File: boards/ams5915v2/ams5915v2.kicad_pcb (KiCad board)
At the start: 2 copper layers, 20 x 56.5 mm, 32 parts, among them J1 Conn_01x04, M3 MountingHole_3.2mm_M3, U1 TLV73333PDBVR, U2 MAX4995A, U3 AMS5915, U4 MAX4995A, U5 AMS5915

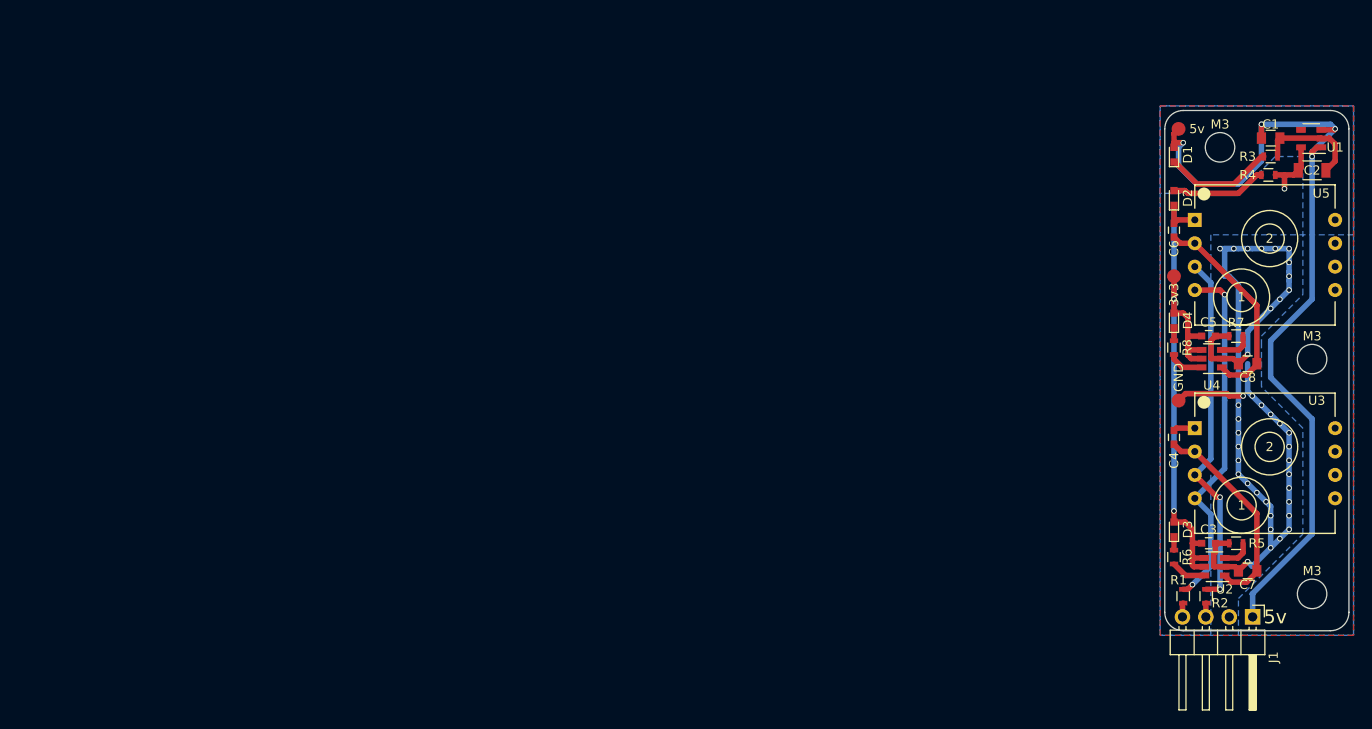
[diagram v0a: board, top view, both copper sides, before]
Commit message: [ams5915v2] new board design
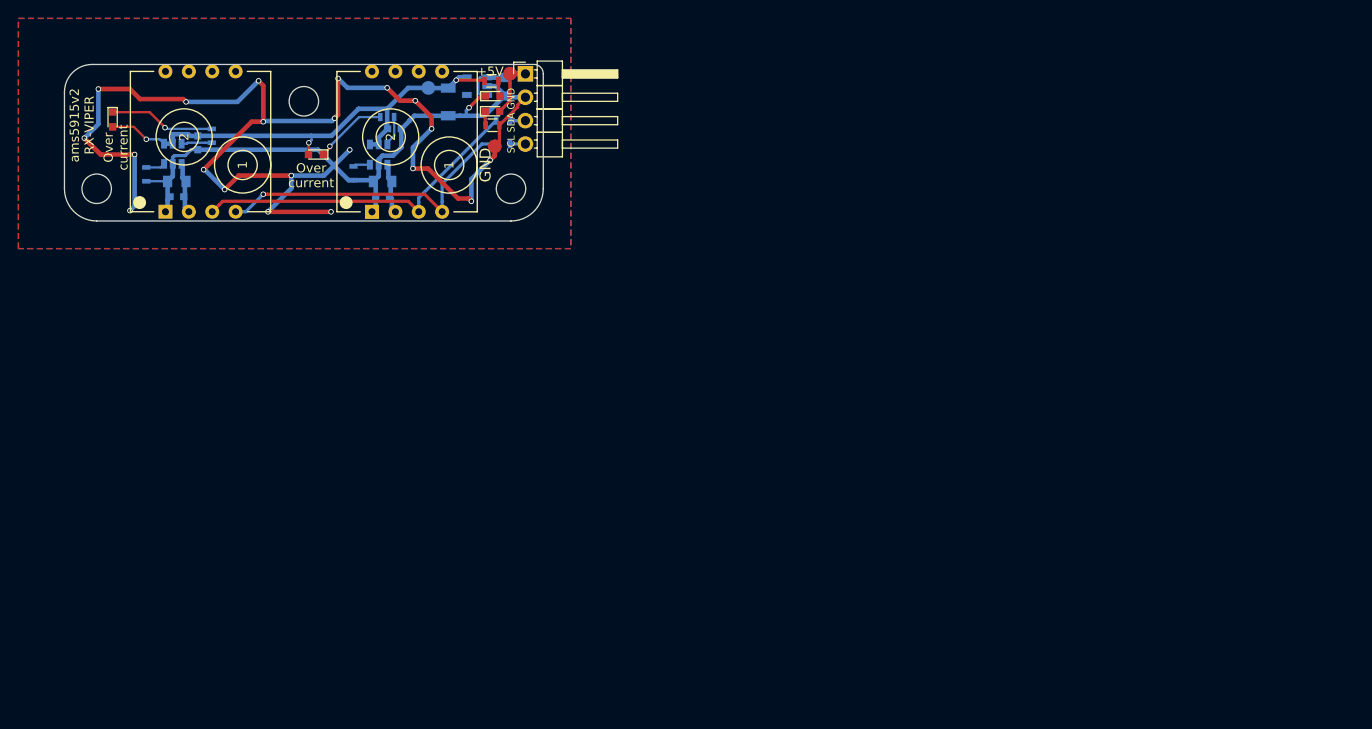
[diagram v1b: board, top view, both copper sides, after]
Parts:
- removed 3v3: 3v3, Measurement_Points:Measurement_Point_Round-SMD-Pad_Small
- removed 5v: 5v, Measurement_Points:Measurement_Point_Round-SMD-Pad_Small
- removed GND: GND, Measurement_Points:Measurement_Point_Round-SMD-Pad_Small
- removed M3 (x3): MountingHole_3.2mm_M3, Mounting_Holes:MountingHole_3.2mm_M3
- added REF**: MountingHole_3.2mm_M3, Mounting_Holes:MountingHole_3.2mm_M3, F.Cu at (60.5, 77.5)
- added REF**: MountingHole_3.2mm_M3, Mounting_Holes:MountingHole_3.2mm_M3, F.Cu at (83.0, 68.0)
- added REF**: MountingHole_3.2mm_M3, Mounting_Holes:MountingHole_3.2mm_M3, F.Cu at (105.5, 77.5)
- added TP1: 5v, Measurement_Points:Measurement_Point_Round-SMD-Pad_Small, F.Cu at (105.4, 65.0)
- added TP2: GND, Measurement_Points:Measurement_Point_Round-SMD-Pad_Small, F.Cu at (103.7, 72.9)
- added TP3: 3v3, Measurement_Points:Measurement_Point_Round-SMD-Pad_Small, B.Cu at (96.5, 66.5)
- C1, C2, C3, C4, C5, C6, C7, C8, R1, R2, R5, R6, R7, R8, U1, U2, U4: moved to B.Cu
- moved R7 119.7 mm to (65.9, 75.9), turned to 90 degrees
- moved C8 118.0 mm to (69.2, 76.7)
- moved D4 117.3 mm to (62.2, 70.0), turned to 270 degrees
- moved U5 115.6 mm to (64.2, 80.0), turned to 0 degrees
- moved U4 115.0 mm to (68.8, 73.7), turned to 90 degrees
- moved C5 111.8 mm to (71.5, 72.5), turned to 270 degrees
- moved C6 108.3 mm to (69.2, 78.4), turned to 180 degrees
- moved R8 107.0 mm to (73.0, 71.7)
- moved R5 103.9 mm to (88.4, 75.8), turned to 90 degrees
- moved C7 103.0 mm to (91.6, 76.7)
- moved D3 101.7 mm to (84.3, 73.8), turned to 180 degrees
- moved U2 101.2 mm to (91.1, 73.8), turned to 90 degrees
- moved C3 99.2 mm to (92.8, 71.0)
- moved J1 98.6 mm to (107.1, 65.0), turned to 0 degrees
- moved R6 97.9 mm to (92.1, 69.7), turned to 0 degrees
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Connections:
- net /5v renamed +5V
- net /GND renamed GND
- U1 pad 4: Net-(U1-Pad4) -> (no net)
- U3 pad 5: Net-(U3-Pad5) -> (no net)
- U3 pad 6: Net-(U3-Pad6) -> (no net)
- U3 pad 7: Net-(U3-Pad7) -> (no net)
- U3 pad 8: Net-(U3-Pad8) -> (no net)
- U5 pad 5: Net-(U5-Pad5) -> (no net)
- U5 pad 6: Net-(U5-Pad6) -> (no net)
- U5 pad 7: Net-(U5-Pad7) -> (no net)
- U5 pad 8: Net-(U5-Pad8) -> (no net)
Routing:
- net +5V: track 94.2 -> 14.1 mm, vias 4 -> 0
- net GND: track 126.4 -> 197.9 mm, vias 39 -> 22
- net Net-(C6-Pad1): track 23.1 -> 5.72 mm
- net Net-(C4-Pad1): track 22.7 -> 5.68 mm
- net /3v3: track 64.9 -> 53.5 mm
- net Net-(D1-Pad1): track 12.0 -> 1.55 mm
- net Net-(D4-Pad1): track 1.40 -> 11.5 mm, vias 0 -> 1
- net Net-(D2-Pad2): track 10.5 -> 1.72 mm
- net Net-(D3-Pad1): track 1.25 -> 7.98 mm, vias 0 -> 1
- net Net-(R1-Pad2): track 39.0 -> 34.7 mm, vias 2 -> 1
- net Net-(R2-Pad2): track 39.3 -> 36.8 mm, vias 2 -> 0
- net Net-(R7-Pad2): track 3.54 -> 2.09 mm
- net Net-(R5-Pad2): track 3.28 -> 1.86 mm
- net Net-(R8-Pad2): track 3.87 -> 3.33 mm
- net Net-(R6-Pad2): track 3.82 -> 3.28 mm
- removed copper zone on B.Cu, net +5V
- removed copper zone on B.Cu, net /3v3
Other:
- board size 20 x 56.5 mm -> 52 x 17 mm
- net class Default: trace_width 0.6 -> 0.25
- board text added: "+3V3"
- board text added: "+5V"
- board text added: "GND"
- board text added: "Over current"
- board text added: "SCL SDA GND"
- board text added: "ams5915v2 RX-VIPER"
- board text removed: "5v"
